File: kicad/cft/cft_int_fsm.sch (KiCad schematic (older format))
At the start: 16 parts, among them U801 74HC74, U802 74LVC1G08, U803 74HC74, U804 74LVC1G32, U805 74HC74

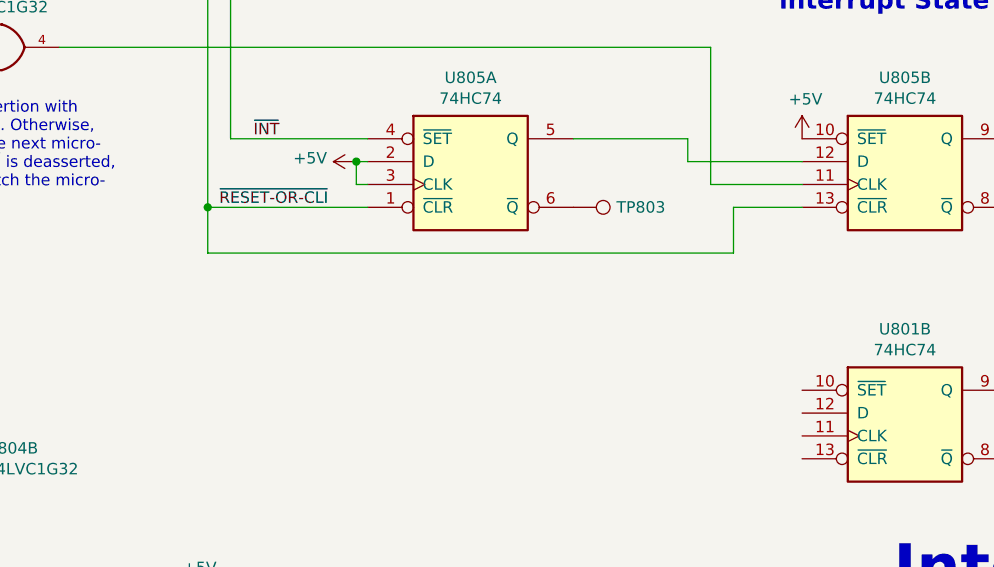
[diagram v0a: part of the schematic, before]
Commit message: Cleaned up Interrupt FSM schematics
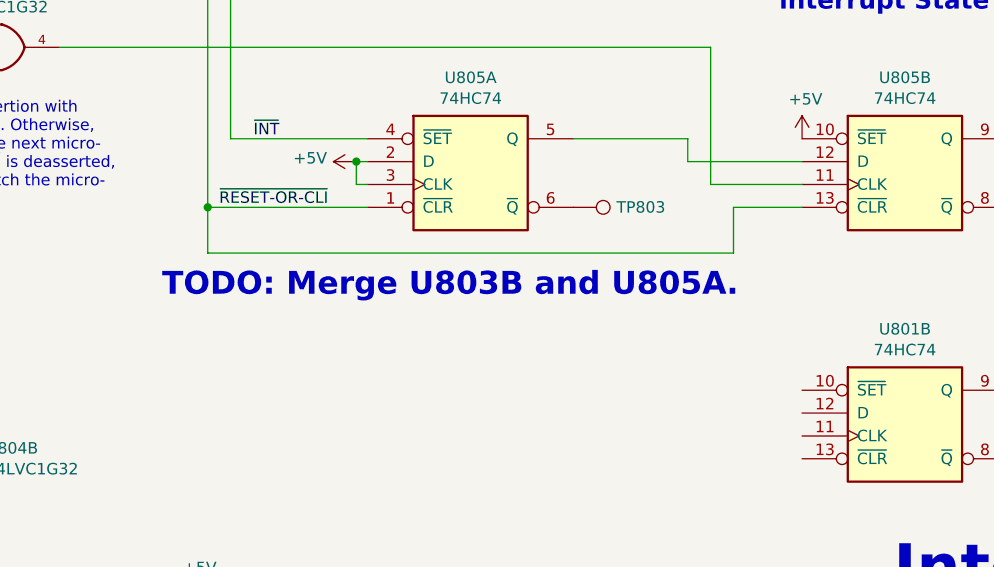
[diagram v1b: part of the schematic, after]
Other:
- note added: "TODO: Merge U803B and U805A."
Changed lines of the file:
@@
 ~IRQS
-$Comp
-L Connector:TestPoint TP802
-U 1 1 5F9307F3
-P 5750 3150
-F 0 "TP802" V 5750 3338 50  0000 L CNN
-F 1 "TestPoint" H 5808 3177 50  0001 L CNN
-F 2 "TestPoint:TestPoint_Keystone_5010-5014_Multipurpose" H 5950 3150 50  0001 C CNN
-F 3 "~" H 5950 3150 50  0001 C CNN
-	1    5750 3150
-	0    1    1    0
-$EndComp
 $Comp
 L Connector:TestPoint TP804
@@
 F 1 "74HC74" H 5300 1976 50  0000 C CNN
 F 2 "Package_SO:SOIC-14_3.9x8.7mm_P1.27mm" H 5300 1650 50  0001 C CNN
-F 3 "74xx/74hc_hct74.pdf" H 5300 1650 50  0001 C CNN
+F 3 "https://assets.nexperia.com/documents/data-sheet/74HC_HCT74.pdf" H 5300 1650 50  0001 C CNN
 	1    5300 1650
 	1    0    0    -1
@@
 F 1 "74HC74" H 5300 3326 50  0000 C CNN
 F 2 "Package_SO:SOIC-14_3.9x8.7mm_P1.27mm" H 5300 3000 50  0001 C CNN
-F 3 "74xx/74hc_hct74.pdf" H 5300 3000 50  0001 C CNN
+F 3 "https://assets.nexperia.com/documents/data-sheet/74HC_HCT74.pdf" H 5300 3000 50  0001 C CNN
 	1    5300 3000
 	1    0    0    -1
@@
 F 1 "74HC74" H 7200 5426 50  0000 C CNN
 F 2 "Package_SO:SOIC-14_3.9x8.7mm_P1.27mm" H 7200 5100 50  0001 C CNN
-F 3 "74xx/74hc_hct74.pdf" H 7200 5100 50  0001 C CNN
+F 3 "https://assets.nexperia.com/documents/data-sheet/74HC_HCT74.pdf" H 7200 5100 50  0001 C CNN
 	2    7200 5100
 	1    0    0    -1
 $EndComp
-Wire Wire Line
-	4850 2850 4250 2850
-Wire Wire Line
-	4250 2850 4250 2300
 Wire Wire Line
 	4250 2300 6250 2300
@@
 Text HLabel 2200 2950 0    50   Input ~ 0
 ~IRQ
-Wire Wire Line
-	5750 2850 6150 2850
-Wire Wire Line
-	6150 2850 6150 2950
 Wire Wire Line
 	6150 2950 6700 2950
@@
 	2200 1750 3000 1750
 $Comp
-L power:+5V #PWR0813
-U 1 1 5D1C81EC
-P 4800 3150
-F 0 "#PWR0813" H 4800 3000 50  0001 C CNN
-F 1 "+5V" V 4815 3278 50  0000 L CNN
-F 2 "" H 4800 3150 50  0001 C CNN
-F 3 "" H 4800 3150 50  0001 C CNN
-	1    4800 3150
-	0    -1   -1   0
-$EndComp
-$Comp
 L power:+5V #PWR0815
 U 1 1 5D1C8231
@@
 F 1 "74HC74" H 5300 5426 50  0000 C CNN
 F 2 "Package_SO:SOIC-14_3.9x8.7mm_P1.27mm" H 5300 5100 50  0001 C CNN
-F 3 "74xx/74hc_hct74.pdf" H 5300 5100 50  0001 C CNN
+F 3 "https://assets.nexperia.com/documents/data-sheet/74HC_HCT74.pdf" H 5300 5100 50  0001 C CNN
 	1    5300 5100
 	1    0    0    -1
@@
 $EndComp
 Connection ~ 4800 5050
-Wire Wire Line
-	4800 3150 4850 3150
 Text Label 4200 5250 0    50   ~ 0
 ~RESET-OR-CLI
@@
 Text Label 4350 2300 0    50   ~ 0
 IRQEN
-Text Label 4350 2850 0    50   ~ 0
-FI
 Text Label 4350 2950 0    50   ~ 0
 ~IRQ
@@
 	1    0    0    -1
 $EndComp
-Text Label 5800 2850 0    50   ~ 0
-~INT₀
 Text Notes 6500 1700 0    50   ~ 0
 This is the Interrupt Flag (interrupt handling enabled)\ndisplayed on the front panel.
@@
 F 1 "74HC74" H 1730 7055 50  0000 L CNN
 F 2 "Package_SO:SOIC-14_3.9x8.7mm_P1.27mm" H 1550 7100 50  0001 C CNN
-F 3 "74xx/74hc_hct74.pdf" H 1550 7100 50  0001 C CNN
+F 3 "https://assets.nexperia.com/documents/data-sheet/74HC_HCT74.pdf" H 1550 7100 50  0001 C CNN
 	3    1550 7100
 	1    0    0    -1
@@
 F 1 "74HC74" H 3180 7055 50  0000 L CNN
 F 2 "Package_SO:SOIC-14_3.9x8.7mm_P1.27mm" H 3000 7100 50  0001 C CNN
-F 3 "74xx/74hc_hct74.pdf" H 3000 7100 50  0001 C CNN
+F 3 "https://assets.nexperia.com/documents/data-sheet/74HC_HCT74.pdf" H 3000 7100 50  0001 C CNN
 	3    3000 7100
 	1    0    0    -1
@@
 F 1 "74HC74" H 4630 7055 50  0000 L CNN
 F 2 "Package_SO:SOIC-14_3.9x8.7mm_P1.27mm" H 4450 7100 50  0001 C CNN
-F 3 "74xx/74hc_hct74.pdf" H 4450 7100 50  0001 C CNN
+F 3 "https://assets.nexperia.com/documents/data-sheet/74HC_HCT74.pdf" H 4450 7100 50  0001 C CNN
 	3    4450 7100
 	1    0    0    -1
@@
 F 1 "74HC74" H 7150 3326 50  0000 C CNN
 F 2 "Package_SO:SOIC-14_3.9x8.7mm_P1.27mm" H 7150 3000 50  0001 C CNN
-F 3 "74xx/74hc_hct74.pdf" H 7150 3000 50  0001 C CNN
+F 3 "https://assets.nexperia.com/documents/data-sheet/74HC_HCT74.pdf" H 7150 3000 50  0001 C CNN
 	2    7150 3000
 	1    0    0    -1
@@
 F 1 "74HC74" H 7200 6526 50  0000 C CNN
 F 2 "Package_SO:SOIC-14_3.9x8.7mm_P1.27mm" H 7200 6200 50  0001 C CNN
-F 3 "74xx/74hc_hct74.pdf" H 7200 6200 50  0001 C CNN
+F 3 "https://assets.nexperia.com/documents/data-sheet/74HC_HCT74.pdf" H 7200 6200 50  0001 C CNN
 	2    7200 6200
 	1    0    0    -1
@@
 Text Notes 8500 6250 0    50   ~ 0
 ~IRQS~ and ~IRQµC~ are the same signal.\nThe former is output to the bus. The latter is\nfor the Microcode Store. We drive them separately\nto keep the capacitance down and because the one going\nto the Microcode Store is more important and must be\nless loaded (and thus rise faster).\n\nTODO: Drive ~IRQSµC using the leftover FF.
+Wire Wire Line
+	6150 2850 6150 2950
+Text Label 5800 2850 0    50   ~ 0
+~INT₀
+Wire Wire Line
+	5750 2850 6150 2850
+$Comp
+L Connector:TestPoint TP802
+U 1 1 5F9307F3
+P 5750 3150
+F 0 "TP802" V 5750 3338 50  0000 L CNN
+F 1 "TestPoint" H 5808 3177 50  0001 L CNN
+F 2 "TestPoint:TestPoint_Keystone_5010-5014_Multipurpose" H 5950 3150 50  0001 C CNN
+F 3 "~" H 5950 3150 50  0001 C CNN
+	1    5750 3150
+	0    1    1    0
+$EndComp
+Wire Wire Line
+	4250 2850 4250 2300
+Text Label 4350 2850 0    50   ~ 0
+FI
+Wire Wire Line
+	4850 2850 4250 2850
+Wire Wire Line
+	4800 3150 4850 3150
+$Comp
+L power:+5V #PWR0813
+U 1 1 5D1C81EC
+P 4800 3150
+F 0 "#PWR0813" H 4800 3000 50  0001 C CNN
+F 1 "+5V" V 4815 3278 50  0000 L CNN
+F 2 "" H 4800 3150 50  0001 C CNN
+F 3 "" H 4800 3150 50  0001 C CNN
+	1    4800 3150
+	0    -1   -1   0
+$EndComp
+Text Notes 3950 5650 0    100  ~ 20
+TODO: Merge U803B and U805A.
 $EndSCHEMATC
